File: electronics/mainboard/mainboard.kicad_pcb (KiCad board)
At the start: 2 copper layers, 151.1 x 55.9 mm, 53 parts, among them J1 Conn_01x09, J10 Conn_01x08, J11 Conn_01x08, J12 Conn_01x08, J13 Conn_02x18_Odd_Even, J14 Conn_01x08, J15 Conn_01x08, J16 Conn_01x10, J17 Conn_02x03_Odd_Even, J2 Conn_01x09, J3 Conn_01x09, J4 Conn_01x09, J5 Conn_01x09, J6 Conn_01x09, J7 Conn_01x09, J8 Conn_01x09, J9 Conn_01x09

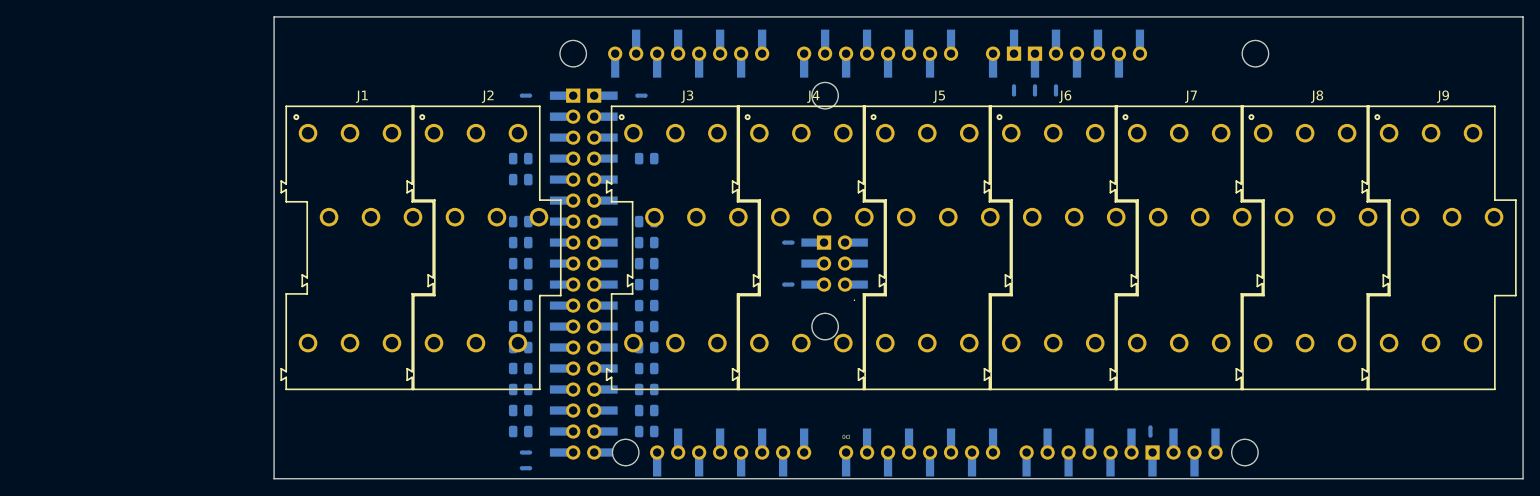
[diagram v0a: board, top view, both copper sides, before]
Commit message: route pcb
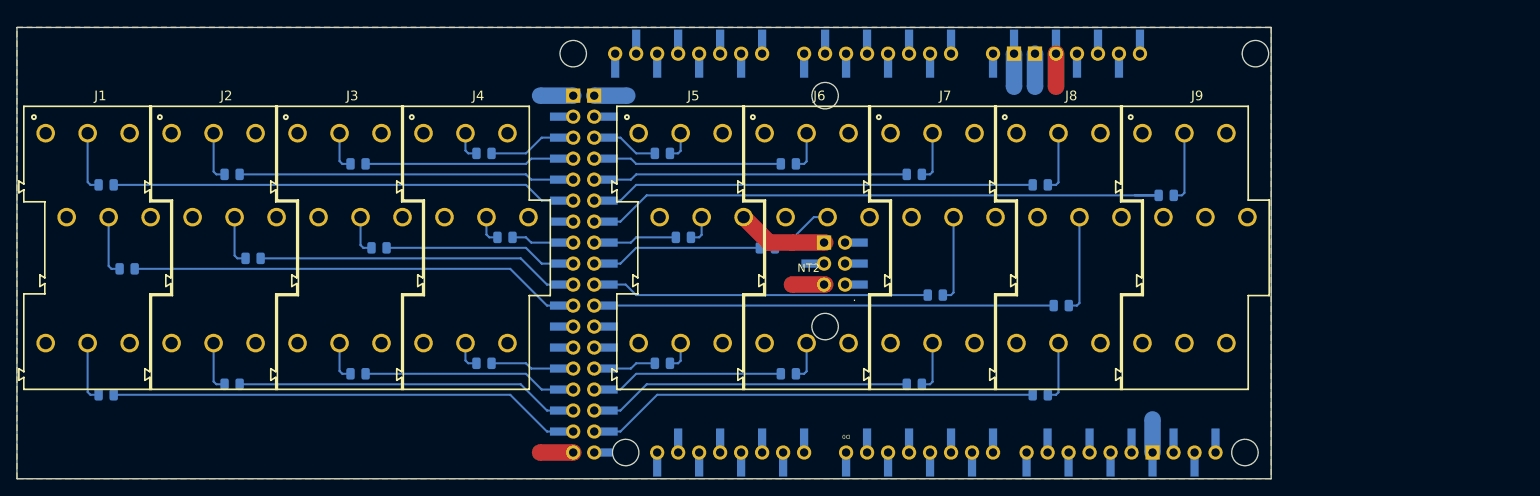
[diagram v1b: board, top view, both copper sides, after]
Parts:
- removed NT10: NetTie_2, NetTie:NetTie-2_SMD_Pad0.5mm
- NT1, NT2, NT3, NT7: footprint NetTie:NetTie-2_SMD_Pad0.5mm -> NetTie:NetTie-2_SMD_Pad2.0mm; moved to F.Cu
- NT4, NT5, NT6, NT8, NT9: footprint NetTie:NetTie-2_SMD_Pad0.5mm -> NetTie:NetTie-2_SMD_Pad2.0mm
- moved R25 78.2 mm to (186.7, 82.5), turned to 180 degrees
- moved NT4 75.8 mm to (185.0, 111.7), turned to -90 degrees
- moved R1 71.9 mm to (58.4, 81.3), turned to 0 degrees
- moved R23 67.2 mm to (174.0, 95.9), turned to 180 degrees
- moved R3 65.4 mm to (58.4, 106.7), turned to 0 degrees
- moved R22 63.0 mm to (171.4, 81.3), turned to 180 degrees
- moved R24 55.5 mm to (171.4, 106.7)
- moved R2 51.5 mm to (61.0, 91.4)
- moved R20 50.6 mm to (158.8, 94.6), turned to 180 degrees
- moved R5 50.2 mm to (76.2, 90.2), turned to 0 degrees
- moved NT5 45.9 mm to (170.8, 67.4), turned to 90 degrees
- moved R4 45.1 mm to (73.7, 80.0)
- moved R7 42.8 mm to (88.9, 78.7), turned to 0 degrees
- moved J4 40.6 mm to (104.4, 85.2)
- moved J3 40.6 mm to (89.2, 85.2)
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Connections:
- NT3 pad 2: /5V3 -> /5V4
- NT4 pad 1: +5V -> GND
- NT4 pad 2: /5V4 -> /GND1
- NT5 pad 2: /GND1 -> /GND2
- NT6 pad 2: /GND2 -> /GND3
- NT7 pad 2: /GND3 -> /GND4
- NT8 pad 2: /GND4 -> /GND5
- NT9 pad 2: /GND5 -> /GND6
- R1 pad 2: /D22 -> /D45
- R10 pad 2: /D31 -> /D51
- R11 pad 2: /D32 -> /D41
- R12 pad 2: /D33 -> /D29
- R13 pad 2: /D34 -> /D50
- R14 pad 2: /D35 -> /D40
- R15 pad 2: /D36 -> /D28
- R16 pad 2: /D37 -> /D48
- R18 pad 2: /D39 -> /D26
- R19 pad 2: /D40 -> /D46
- R2 pad 2: /D23 -> /D35
- R20 pad 2: /D41 -> /D36
- R21 pad 2: /D42 -> /D24
- R22 pad 2: /D43 -> /D44
- R23 pad 2: /D47 -> /D34
- R24 pad 2: /D48 -> /D22
- R25 pad 2: /D49 -> /D42
- R3 pad 2: /D24 -> /D23
- R4 pad 2: /D25 -> /D47
- R5 pad 2: /D26 -> /D37
- R6 pad 2: /D27 -> /D25
- R7 pad 2: /D28 -> /D49
- R8 pad 2: /D29 -> /D39
- R9 pad 2: /D30 -> /D27
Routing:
- net /D42: track 0.00 -> 72.2 mm
- net /D23: track 0.00 -> 57.4 mm
- net /D45: track 0.00 -> 56.4 mm
- net /D34: track 0.00 -> 55.6 mm
- net /D35: track 0.00 -> 54.9 mm
- net /D44: track 0.00 -> 53.9 mm
- net /D22: track 0.00 -> 53.6 mm
- net /D25: track 0.00 -> 41.7 mm
- net /D36: track 0.00 -> 40.9 mm
- net /D47: track 0.00 -> 40.6 mm
- net /D24: track 0.00 -> 39.1 mm
- net /D37: track 0.00 -> 39.1 mm
- net /D46: track 0.00 -> 38.1 mm
- net /D27: track 0.00 -> 25.9 mm
- net /D49: track 0.00 -> 25.4 mm
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- added copper zone on F.Cu, net +5V
- added copper zone on B.Cu, net GND
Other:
- board size 151.1 x 55.9 mm -> 151.8 x 54.6 mm
